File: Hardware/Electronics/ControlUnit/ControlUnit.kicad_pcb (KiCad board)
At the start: 2 copper layers, 1 part

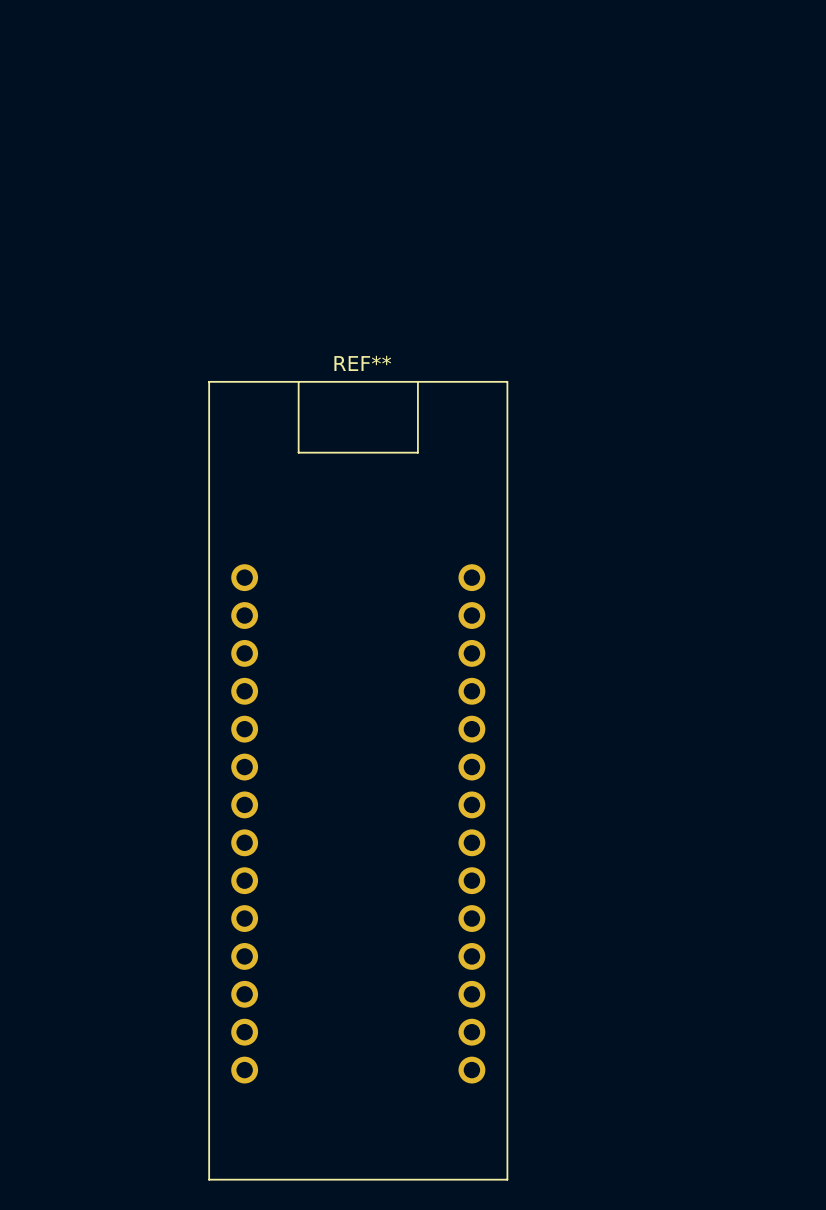
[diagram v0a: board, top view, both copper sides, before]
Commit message: Encore
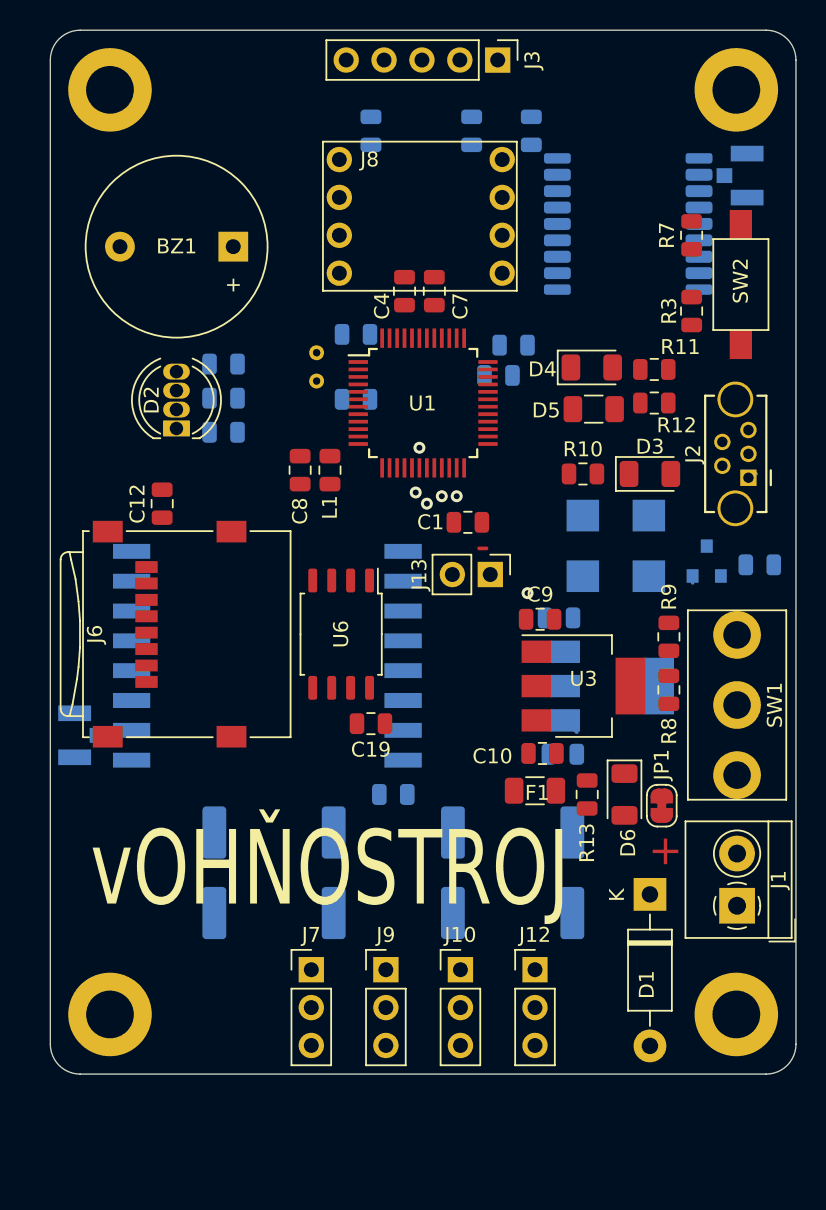
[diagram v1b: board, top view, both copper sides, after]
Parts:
- removed REF**: RobotDyn_SAMD21_M0-Mini, CustomLib:RobotDyn_SAMD21_M0-Mini
- added BZ1: Buzzer, Buzzer_Beeper:Buzzer_12x9.5RM7.6, F.Cu at (112.3, 64.5)
- added C1: 100nF, Capacitor_SMD:C_0805_2012Metric, F.Cu at (128.0, 83.0)
- added C10: 10uF, Capacitor_SMD:C_0805_2012Metric, F.Cu at (133.0, 98.5)
- added C11: 100nF, Capacitor_SMD:C_0805_2012Metric, B.Cu at (123.0, 101.2)
- added C12: 100nF, Capacitor_SMD:C_0805_2012Metric, F.Cu at (107.5, 81.8)
- added C13: 100nF, Capacitor_SMD:C_0805_2012Metric, B.Cu at (132.2, 56.8)
- added C14: 100nF, Capacitor_SMD:C_0805_2012Metric, B.Cu at (121.5, 56.8)
- added C15: 100uF, Capacitor_SMD:CP_Elec_6.3x7.7, B.Cu at (111.0, 106.5)
- added C16: 100nF, Capacitor_SMD:C_0805_2012Metric, B.Cu at (128.2, 56.8)
- added C17: 100uF, Capacitor_SMD:CP_Elec_6.3x7.7, B.Cu at (119.0, 106.5)
- added C18: 100uF, Capacitor_SMD:CP_Elec_6.3x7.7, B.Cu at (127.0, 106.5)
- added C19: 100nF, Capacitor_SMD:C_0805_2012Metric, F.Cu at (121.5, 96.5)
- added C2: 12pF, Capacitor_SMD:C_0805_2012Metric, B.Cu at (120.5, 70.4)
- added C20: 100uF, Capacitor_SMD:CP_Elec_6.3x7.7, B.Cu at (135.0, 106.5)
- added C3: 12pF, Capacitor_SMD:C_0805_2012Metric, B.Cu at (120.5, 74.8)
- added C4: 100nF, Capacitor_SMD:C_0805_2012Metric, F.Cu at (123.8, 67.5)
- added C5: 220nF, Capacitor_SMD:C_0805_2012Metric, B.Cu at (134.4, 98.6)
- added C6: 100nF, Capacitor_SMD:C_0805_2012Metric, B.Cu at (134.1, 89.4)
- added C7: 1uF, Capacitor_SMD:C_0805_2012Metric, F.Cu at (125.8, 67.5)
- added C8: 100nF, Capacitor_SMD:C_0805_2012Metric, F.Cu at (116.8, 79.5)
- added C9: 1uF, Capacitor_SMD:C_0805_2012Metric, F.Cu at (132.8, 89.5)
- added D1: D, Diode_THT:D_DO-41_SOD81_P10.16mm_Horizontal, F.Cu at (140.2, 108.0)
- added D2: LED_RCGB, LED_THT:LED_D5.0mm-4_RGB, F.Cu at (108.5, 76.7)
- added D3: LED, LED_SMD:LED_1206_3216Metric, F.Cu at (140.2, 79.8)
- added D4: LED, LED_SMD:LED_1206_3216Metric, F.Cu at (136.3, 72.6)
- added D5: LED, Fuse:Fuse_1206_3216Metric, F.Cu at (136.4, 75.4)
- added D6: LED, LED_SMD:LED_1206_3216Metric, F.Cu at (138.5, 101.2)
- added D7: D_Schottky, CustomLib:DIOM5436X244N, B.Cu at (137.9, 82.5)
- added D8: D_Schottky, CustomLib:DIOM5436X244N, B.Cu at (137.9, 86.6)
- added F1: 500mA, Fuse:Fuse_1206_3216Metric, F.Cu at (132.5, 101.0)
- added H1: MountingHole, MountingHole:MountingHole_3.2mm_M3_DIN965_Pad, F.Cu at (104.0, 54.0)
- added H2: MountingHole, MountingHole:MountingHole_3.2mm_M3_DIN965_Pad, F.Cu at (146.0, 54.0)
- added H3: MountingHole, MountingHole:MountingHole_3.2mm_M3_DIN965_Pad, F.Cu at (104.0, 116.0)
- added H4: MountingHole, MountingHole:MountingHole_3.2mm_M3_DIN965_Pad, F.Cu at (146.0, 116.0)
- added J1: Screw_Terminal_01x02, Batt 9V, TerminalBlock_4Ucon:TerminalBlock_4Ucon_1x02_P3.50mm_Horizontal, F.Cu at (146.1, 108.7)
- added J10: S3, Connector_PinHeader_2.54mm:PinHeader_1x03_P2.54mm_Vertical, F.Cu at (127.5, 113.0)
- added J11: MPU-6050/MPU-9250, Switch:MPU-9250-4pin, B.Cu at (130.3, 58.7)
- added J12: S4, Connector_PinHeader_2.54mm:PinHeader_1x03_P2.54mm_Vertical, F.Cu at (132.5, 113.0)
- added J13: Conn_01x02, Connector_PinHeader_2.54mm:PinHeader_1x02_P2.54mm_Vertical, F.Cu at (129.5, 86.5)
- added J2: USB_B_Mini, Connector_USB:USB_Mini-B_Tensility_54-00023_Vertical_CircularHoles, F.Cu at (146.8, 80.0)
- added J3: Conn_01x05, Connector_PinHeader_2.54mm:PinHeader_1x05_P2.54mm_Vertical, F.Cu at (130.0, 52.0)
- added J4: Conn_Coaxial, Connector_Coaxial:U.FL_Hirose_U.FL-R-SMT-1_Vertical, B.Cu at (102.1, 97.3)
- added J5: Conn_Coaxial, Connector_Coaxial:U.FL_Hirose_U.FL-R-SMT-1_Vertical, B.Cu at (146.2, 59.8)
- added J6: Micro_SD_Card, Connector_Card:microSD_HC_Wuerth_693072010801, F.Cu at (108.0, 90.5)
- added J7: S1, Connector_PinHeader_2.54mm:PinHeader_1x03_P2.54mm_Vertical, F.Cu at (117.5, 113.0)
- added J8: BME280, CustomLib:BME280, F.Cu at (119.4, 58.7)
- added J9: S2, Connector_PinHeader_2.54mm:PinHeader_1x03_P2.54mm_Vertical, F.Cu at (122.5, 113.0)
- added JP1: SolderJumper_2_Bridged, Jumper:SolderJumper-2_P1.3mm_Bridged_RoundedPad1.0x1.5mm, F.Cu at (141.0, 102.0)
- added L1: 10uH, Inductor_SMD:L_0805_2012Metric, F.Cu at (118.8, 79.5)
- added Q1: BSH203, Package_TO_SOT_SMD:SOT-23, B.Cu at (144.0, 85.6)
- added R1: 10k, Resistor_SMD:R_0805_2012Metric, B.Cu at (130.0, 73.2)
- added R10: R, Resistor_SMD:R_0805_2012Metric, F.Cu at (135.7, 79.8)
- added R11: R, Resistor_SMD:R_0805_2012Metric, F.Cu at (140.5, 72.8)
- added R12: R, Resistor_SMD:R_0805_2012Metric, F.Cu at (140.5, 75.0)
- added R13: R, Resistor_SMD:R_0805_2012Metric, F.Cu at (136.0, 101.2)
- added R14: 10k, Resistor_SMD:R_0805_2012Metric, B.Cu at (147.6, 85.9)
- added R2: 10k, Resistor_SMD:R_0805_2012Metric, B.Cu at (131.1, 71.1)
- added R3: 10k, Resistor_SMD:R_0805_2012Metric, F.Cu at (143.0, 68.8)
- added R4: 220, Resistor_SMD:R_0805_2012Metric, B.Cu at (111.6, 77.0)
- added R5: 220, Resistor_SMD:R_0805_2012Metric, B.Cu at (111.6, 74.7)
- added R6: 220, Resistor_SMD:R_0805_2012Metric, B.Cu at (111.6, 72.4)
- added R7: 100k, Resistor_SMD:R_0805_2012Metric, F.Cu at (143.0, 63.8)
- added R8: 100k, Resistor_SMD:R_0805_2012Metric, F.Cu at (141.5, 94.2)
- added R9: 100k, Resistor_SMD:R_0805_2012Metric, F.Cu at (141.5, 90.7)
- added SW1: SW_DPDT_x2, Switch:Sw1, F.Cu at (146.1, 95.2)
- added SW2: SW_Push, CustomLib:Push_Switch_TS1107GS-5, F.Cu at (146.3, 67.1)
- added U1: ATSAMD21G18A-AF, Package_QFP:TQFP-48_7x7mm_P0.5mm, F.Cu at (125.0, 75.0)
- added U2: LM340_SOT223/LM7805_5V, Package_TO_SOT_SMD:SOT-223-3_TabPin2, B.Cu at (137.7, 94.0)
- added U3: MCP1826S_3.3V, Package_TO_SOT_SMD:SOT-223-3_TabPin2, F.Cu at (135.8, 94.0)
- added U4: RFM69W, RF_Module:HOPERF_RFM69HW, B.Cu at (114.6, 91.9)
- added U5: MAX-8Q, RF_GPS:ublox_MAX, B.Cu at (138.8, 63.0)
- added U6: W25Q32JVSS, Package_SO:SOIC-8_5.23x5.23mm_P1.27mm, F.Cu at (119.5, 90.5)
- added Y1: 32.768kHz, Crystal:Crystal_C26-LF_D2.1mm_L6.5mm_Horizontal, B.Cu at (117.9, 71.6)
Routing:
- net Net-(D7-Pad2): track 0.00 -> 1.92 mm
- net /Vbatt: track 0.00 -> 1.22 mm
- net /MOSI: track 0.00 -> 0.63 mm, vias 0 -> 1
- net Net-(J13-Pad1): track 0.00 -> 0.50 mm
- net +5V: track 0.00 -> 0.10 mm, vias 0 -> 1
- net GND: vias 0 -> 1
- net /SCK: vias 0 -> 1
- net /MISO: vias 0 -> 1
- net /CS_RAD: vias 0 -> 1
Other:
- board outline added: 50 x 70 mm
- board text added: "+"
- board text added: "vOHŇOSTROJ"
